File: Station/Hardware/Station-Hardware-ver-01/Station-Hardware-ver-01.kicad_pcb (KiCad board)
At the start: 2 copper layers, 55 x 70 mm, 28 parts, among them J1 Barrel_Jack, J2 Conn_01x03_Male, J3 Conn_01x03_Male, J4 4P4C, J5 4P4C, J6 Conn_01x03_Male, U1 YAAJ_BluePill, U2 DS3231_Full_Pinout, U3 SX1278_Minimal, U4 MCP6002-xP, U5 BME280_I2C_New_LK888, U6 LM317_TO-220

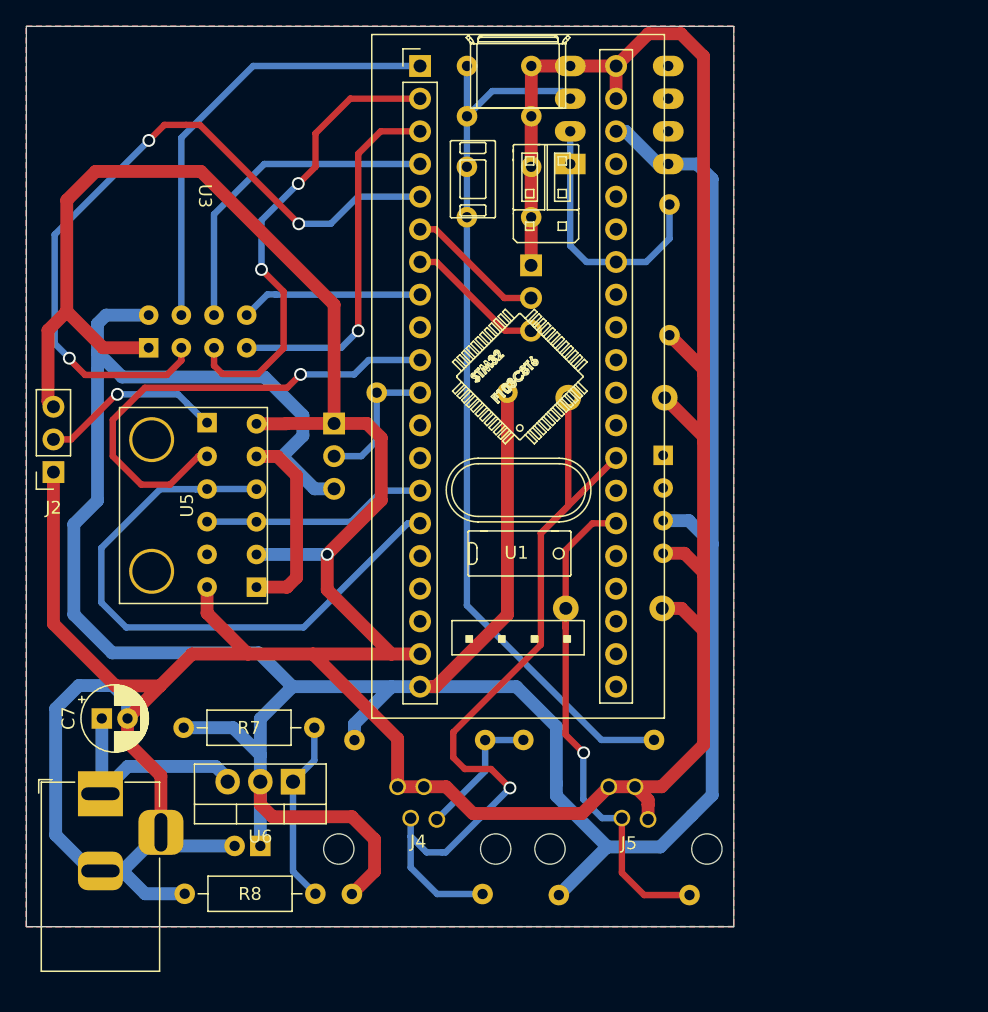
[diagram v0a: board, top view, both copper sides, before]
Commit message: pcb design for the station
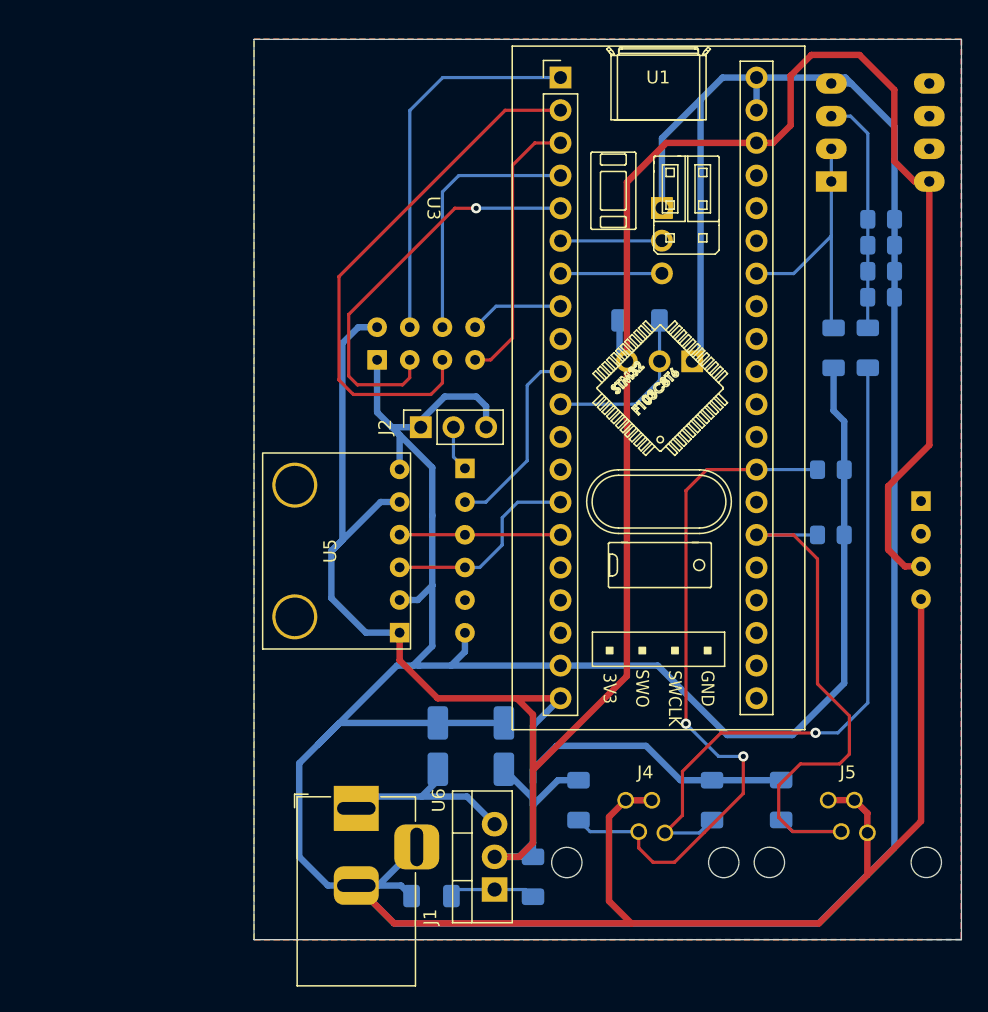
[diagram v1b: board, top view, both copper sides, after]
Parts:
- C1, C6: footprint Capacitor_THT:C_Disc_D8.0mm_W5.0mm_P7.50mm -> Capacitor_SMD:C_0805_2012Metric_Pad1.18x1.45mm_HandSolder
- C2, C3, C4, C5: footprint Capacitor_THT:C_Disc_D5.1mm_W3.2mm_P5.00mm -> Capacitor_SMD:C_0805_2012Metric_Pad1.18x1.45mm_HandSolder
- C7: footprint Capacitor_THT:CP_Radial_D5.0mm_P2.00mm -> Capacitor_SMD:CP_Elec_4x5.4; moved to B.Cu
- C8: footprint Capacitor_THT:CP_Radial_D5.0mm_P2.00mm -> Capacitor_SMD:CP_Elec_4x5.4
- J2: value Conn_01x03_Male -> 32768 Hz
- J3: value Conn_01x03_Male -> UART
- J6: value Conn_01x03_Male -> DS18B20
- R1, R2, R3, R4, R5, R6: footprint Resistor_THT:R_Axial_DIN0207_L6.3mm_D2.5mm_P10.16mm_Horizontal -> Resistor_SMD:R_1206_3216Metric_Pad1.30x1.75mm_HandSolder
- R7, R8: footprint Resistor_THT:R_Axial_DIN0207_L6.3mm_D2.5mm_P10.16mm_Horizontal -> Resistor_SMD:R_1206_3216Metric_Pad1.30x1.75mm_HandSolder; moved to B.Cu
- U1: footprint KiCAD_STM32_BluePill:YAAJ_BluePill_1 -> KiCAD-STM32BluePill:YAAJ_BluePill_1
- U4: value MCP6002-xP -> MCP6002
- U5: value BME280_I2C_New_LK888 -> BME280_I2C
- U6: value LM317_TO-220 -> LM317
- moved R3 40.6 mm to (215.4, 65.0), turned to 90 degrees
- moved C2 36.9 mm to (216.5, 61.1)
- moved C3 34.4 mm to (216.5, 59.0)
- moved C4 32.8 mm to (216.5, 57.0)
- moved C5 32.2 mm to (216.5, 55.0)
- moved J2 28.8 mm to (180.7, 71.2), turned to 90 degrees
- moved J6 28.3 mm to (201.8, 66.0), turned to 90 degrees
- moved R1 28.2 mm to (203.3, 100.2), turned to -90 degrees
- moved C7 26.2 mm to (182.0, 96.0), turned to 90 degrees
- moved R7 20.6 mm to (189.4, 106.1), turned to 90 degrees
- moved C8 20.5 mm to (187.1, 96.0), turned to 90 degrees
- moved U2 20.4 mm to (201.8, 80.7)
- moved U4 20.3 mm to (212.6, 52.1)
- moved J1 19.9 mm to (175.7, 100.8)
- moved R2 19.1 mm to (192.9, 100.2), turned to -90 degrees
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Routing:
- net GND: track 345.8 -> 401.4 mm, vias 1 -> 0
- net /Passive LPF: track 69.9 -> 18.6 mm
- net WindVane_raw: track 10.7 -> 52.1 mm, vias 0 -> 1
- net I2C_SDA: track 48.2 -> 12.5 mm
- net +3V3: track 269.1 -> 240.1 mm
- net LoRa_Reset: track 56.8 -> 31.3 mm, vias 3 -> 1
- net RTC_ALARM: track 37.8 -> 15.1 mm, vias 1 -> 0
- net Anemometer: track 65.9 -> 54.6 mm, vias 1 -> 2
- net /32768Hz out: track 14.3 -> 3.58 mm, vias 1 -> 0
- net /V_adj: track 14.3 -> 6.78 mm
- net LoRa_DIO0: track 14.2 -> 7.32 mm
- net LoRa_MISO: track 28.5 -> 22.1 mm, vias 1 -> 0
- net Rain_Gauge: track 40.1 -> 45.8 mm, vias 1 -> 0
- net LoRa_MOSI: track 25.5 -> 20.2 mm
- net LoRa_NCSS: track 34.7 -> 29.6 mm
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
